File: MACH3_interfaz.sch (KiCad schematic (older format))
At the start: 66 parts, among them J1 USB_B_Micro, J11 Screw_Terminal_01x06, J2 DB25_Male_MountingHoles, J3 Screw_Terminal_01x06, J4 Screw_Terminal_01x13, J5 B4B-XH-A_LF__SN_, J6 B4B-XH-A_LF__SN_, J7 B4B-XH-A_LF__SN_, J8 B4B-XH-A_LF__SN_, J9 B4B-XH-A_LF__SN_, Q1 2N7002, Q2 MMBT2222ALT3G, U1 74HC245, U10 PC817, U2 74HC245, U3 PC817, U4 PC817, U5 PC817, U6 PC817, U7 PC817, U8 LM317MABDTG, U9 LM358

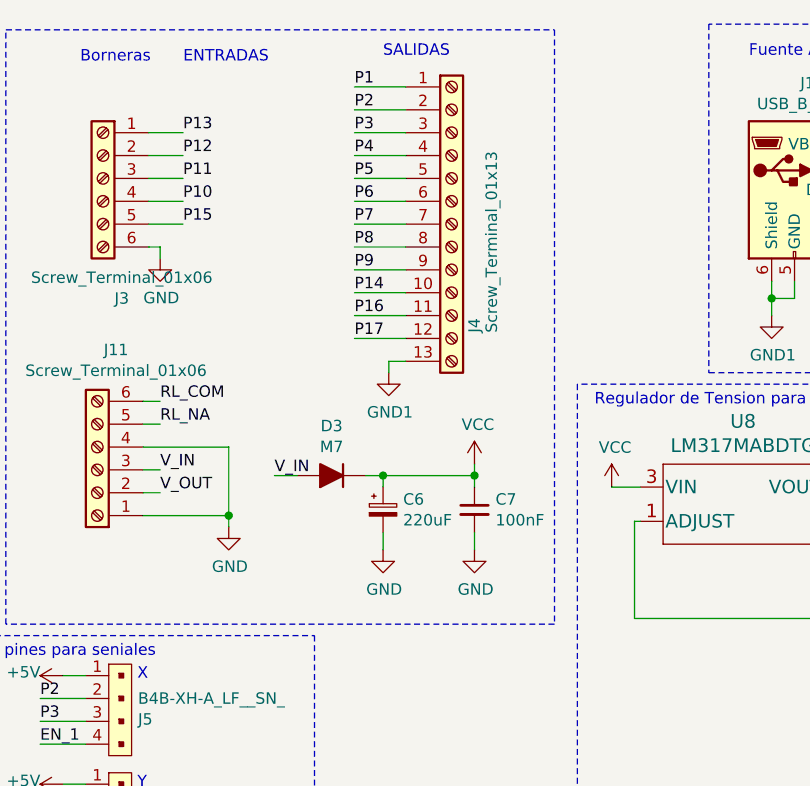
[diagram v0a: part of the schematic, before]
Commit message: Para correccion Docente Eschema, Companiero PCB
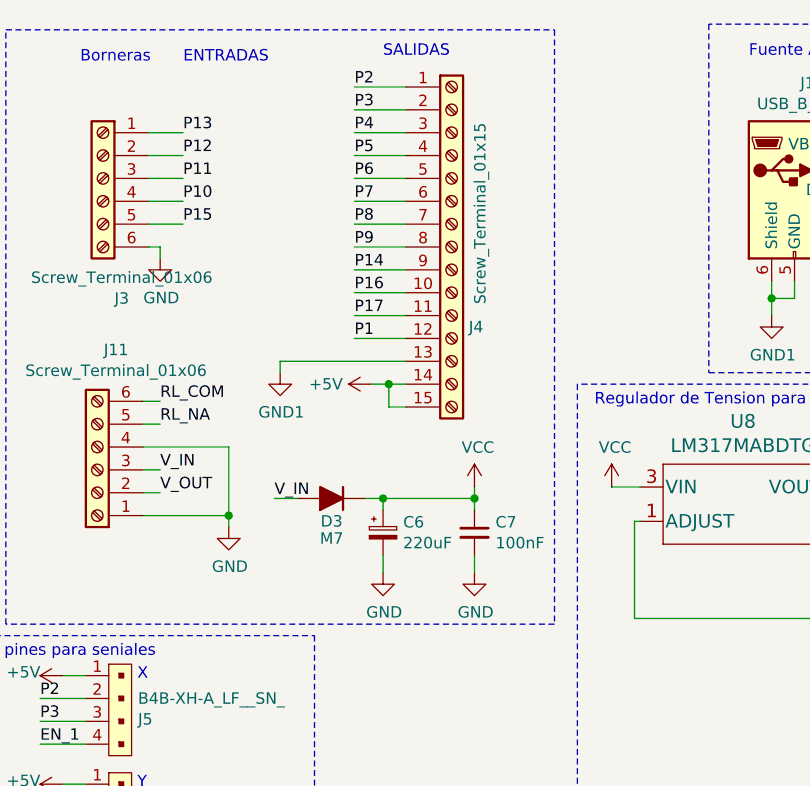
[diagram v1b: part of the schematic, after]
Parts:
- removed J4: Screw_Terminal_01x13, TerminalBlock_Phoenix:TerminalBlock_Phoenix_MKDS-1,5-13_1x13_P5.00mm_Horizontal, symbol Connector:Screw_Terminal_01x13
- added J4: Screw_Terminal_01x15, TerminalBlock_Phoenix:TerminalBlock_Phoenix_MKDS-1,5-15_1x15_P5.00mm_Horizontal, symbol Connector:Screw_Terminal_01x15
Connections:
- net +5V: now also J4.14 (Pin_14), J4.15 (Pin_15)
- net GND1: now also J4.13 (Pin_13)
- net P1: now also J4.12 (Pin_12)
- net P14: now also J4.9 (Pin_9)
- net P16: now also J4.10 (Pin_10)
- net P17: now also J4.11 (Pin_11)
- net P2: now also J4.1 (Pin_1)
- net P3: now also J4.2 (Pin_2)
- net P4: now also J4.3 (Pin_3)
- net P5: now also J4.4 (Pin_4)
- net P6: now also J4.5 (Pin_5)
- net P7: now also J4.6 (Pin_6)
- net P8: now also J4.7 (Pin_7)
- net P9: now also J4.8 (Pin_8)
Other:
- moved on the sheet: C6, C7, D3
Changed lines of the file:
@@
 Text Label 5075 3925 0    50   ~ 0
 P17
-$Comp
-L Connector:Screw_Terminal_01x13 J4
-U 1 1 60736E15
-P 7750 1375
-F 0 "J4" V 7850 900 50  0000 L CNN
-F 1 "Screw_Terminal_01x13" V 7925 900 50  0000 L CNN
-F 2 "TerminalBlock_Phoenix:TerminalBlock_Phoenix_MKDS-1,5-13_1x13_P5.00mm_Horizontal" H 7750 1375 50  0001 C CNN
-F 3 "~" H 7750 1375 50  0001 C CNN
-	1    7750 1375
-	1    0    0    -1
-$EndComp
+Wire Wire Line
+	7550 1875 7325 1875
 Wire Wire Line
 	7550 775  7325 775
@@
 	7550 1775 7325 1775
 Wire Wire Line
-	7550 1875 7325 1875
-Wire Wire Line
-	7550 1975 7475 1975
-Wire Wire Line
-	7475 1975 7475 2025
+	7550 1975 7000 1975
+Wire Wire Line
+	7000 1975 7000 2025
+Text Label 7325 1875 0    50   ~ 0
+P1
 Text Label 7325 775  0    50   ~ 0
-P1
+P2
 Text Label 7325 875  0    50   ~ 0
-P2
+P3
 Text Label 7325 975  0    50   ~ 0
-P3
+P4
 Text Label 7325 1075 0    50   ~ 0
-P4
+P5
 Text Label 7325 1175 0    50   ~ 0
-P5
+P6
 Text Label 7325 1275 0    50   ~ 0
-P6
+P7
 Text Label 7325 1375 0    50   ~ 0
-P7
+P8
 Text Label 7325 1475 0    50   ~ 0
-P8
+P9
 Text Label 7325 1575 0    50   ~ 0
-P9
+P14
 Text Label 7325 1675 0    50   ~ 0
-P14
+P16
 Text Label 7325 1775 0    50   ~ 0
-P16
-Text Label 7325 1875 0    50   ~ 0
 P17
 Text Notes 7450 650  0    50   ~ 0
@@
 $EndComp
 Wire Wire Line
-	7850 2800 7850 2725
+	7850 2900 7850 2825
 $Comp
 L power:GND #PWR0122
 U 1 1 6077A5B8
-P 7850 2800
-F 0 "#PWR0122" H 7850 2550 50  0001 C CNN
-F 1 "GND" H 7855 2627 50  0000 C CNN
-F 2 "" H 7850 2800 50  0001 C CNN
-F 3 "" H 7850 2800 50  0001 C CNN
-	1    7850 2800
-	1    0    0    -1
-$EndComp
-Connection ~ 7450 2475
-Wire Wire Line
-	7850 2475 7450 2475
-Wire Wire Line
-	7850 2525 7850 2475
-Wire Wire Line
-	7450 2475 7450 2525
+P 7850 2900
+F 0 "#PWR0122" H 7850 2650 50  0001 C CNN
+F 1 "GND" H 7855 2727 50  0000 C CNN
+F 2 "" H 7850 2900 50  0001 C CNN
+F 3 "" H 7850 2900 50  0001 C CNN
+	1    7850 2900
+	1    0    0    -1
+$EndComp
+Connection ~ 7450 2575
+Wire Wire Line
+	7850 2575 7450 2575
+Wire Wire Line
+	7850 2625 7850 2575
+Wire Wire Line
+	7450 2575 7450 2625
 $Comp
 L Device:CP_Small C6
 U 1 1 606FAE5F
-P 7450 2625
-F 0 "C6" H 7538 2671 50  0000 L CNN
-F 1 "220uF" H 7538 2580 50  0000 L CNN
-F 2 "Capacitor_THT:CP_Radial_D8.0mm_P3.80mm" H 7450 2625 50  0001 C CNN
-F 3 "~" H 7450 2625 50  0001 C CNN
-	1    7450 2625
+P 7450 2725
+F 0 "C6" H 7538 2771 50  0000 L CNN
+F 1 "220uF" H 7538 2680 50  0000 L CNN
+F 2 "Capacitor_THT:CP_Radial_D8.0mm_P3.80mm" H 7450 2725 50  0001 C CNN
+F 3 "~" H 7450 2725 50  0001 C CNN
+	1    7450 2725
 	1    0    0    -1
 $EndComp
@@
 L power:GND #PWR0123
 U 1 1 6074053C
-P 7450 2800
-F 0 "#PWR0123" H 7450 2550 50  0001 C CNN
-F 1 "GND" H 7455 2627 50  0000 C CNN
-F 2 "" H 7450 2800 50  0001 C CNN
-F 3 "" H 7450 2800 50  0001 C CNN
-	1    7450 2800
-	1    0    0    -1
-$EndComp
-Wire Wire Line
-	7375 2475 7450 2475
+P 7450 2900
+F 0 "#PWR0123" H 7450 2650 50  0001 C CNN
+F 1 "GND" H 7455 2727 50  0000 C CNN
+F 2 "" H 7450 2900 50  0001 C CNN
+F 3 "" H 7450 2900 50  0001 C CNN
+	1    7450 2900
+	1    0    0    -1
+$EndComp
+Wire Wire Line
+	7375 2575 7450 2575
 $Comp
 L Device:D_ALT D3
 U 1 1 606DE50A
-P 7225 2475
-F 0 "D3" H 7225 2258 50  0000 C CNN
-F 1 "M7" H 7225 2349 50  0000 C CNN
-F 2 "Diode_SMD:D_SMA_Handsoldering" H 7225 2475 50  0001 C CNN
-F 3 "~" H 7225 2475 50  0001 C CNN
-	1    7225 2475
+P 7225 2575
+F 0 "D3" H 7225 2675 50  0000 C CNN
+F 1 "M7" H 7225 2750 50  0000 C CNN
+F 2 "Diode_SMD:D_SMA_Handsoldering" H 7225 2575 50  0001 C CNN
+F 3 "~" H 7225 2575 50  0001 C CNN
+	1    7225 2575
 	-1   0    0    1
 $EndComp
@@
 L Device:C_Small C7
 U 1 1 6129BC97
-P 7850 2625
-F 0 "C7" H 7942 2671 50  0000 L CNN
-F 1 "100nF" H 7942 2580 50  0000 L CNN
-F 2 "Capacitor_SMD:C_0805_2012Metric_Pad1.18x1.45mm_HandSolder" H 7850 2625 50  0001 C CNN
-F 3 "~" H 7850 2625 50  0001 C CNN
-	1    7850 2625
+P 7850 2725
+F 0 "C7" H 7942 2771 50  0000 L CNN
+F 1 "100nF" H 7942 2680 50  0000 L CNN
+F 2 "Capacitor_SMD:C_0805_2012Metric_Pad1.18x1.45mm_HandSolder" H 7850 2725 50  0001 C CNN
+F 3 "~" H 7850 2725 50  0001 C CNN
+	1    7850 2725
 	1    0    0    -1
 $EndComp
@@
 L power:GND1 #PWR0105
 U 1 1 626D01A2
-P 7475 2025
-F 0 "#PWR0105" H 7475 1775 50  0001 C CNN
-F 1 "GND1" H 7480 1852 50  0000 C CNN
-F 2 "" H 7475 2025 50  0001 C CNN
-F 3 "" H 7475 2025 50  0001 C CNN
-	1    7475 2025
+P 7000 2025
+F 0 "#PWR0105" H 7000 1775 50  0001 C CNN
+F 1 "GND1" H 7005 1852 50  0000 C CNN
+F 2 "" H 7000 2025 50  0001 C CNN
+F 3 "" H 7000 2025 50  0001 C CNN
+	1    7000 2025
 	1    0    0    -1
 $EndComp
@@
 	9950 3025 9950 2925
 Wire Wire Line
-	7450 2800 7450 2725
+	7450 2900 7450 2825
 Wire Wire Line
 	6475 1475 6475 1525
@@
 L power:VCC #PWR0144
 U 1 1 629C176A
-P 7850 2425
-F 0 "#PWR0144" H 7850 2275 50  0001 C CNN
-F 1 "VCC" H 7865 2598 50  0000 C CNN
-F 2 "" H 7850 2425 50  0001 C CNN
-F 3 "" H 7850 2425 50  0001 C CNN
-	1    7850 2425
+P 7850 2525
+F 0 "#PWR0144" H 7850 2375 50  0001 C CNN
+F 1 "VCC" H 7865 2698 50  0000 C CNN
+F 2 "" H 7850 2525 50  0001 C CNN
+F 3 "" H 7850 2525 50  0001 C CNN
+	1    7850 2525
 	1    0    0    -1
 $EndComp
@@
 $EndComp
 Wire Wire Line
-	7850 2425 7850 2475
-Connection ~ 7850 2475
+	7850 2525 7850 2575
+Connection ~ 7850 2575
 $Comp
 L power:VCC #PWR0146
@@
 	6400 2450 6475 2450
 Wire Wire Line
-	7075 2475 6975 2475
+	7075 2575 6975 2575
 Text Label 6475 2450 0    50   ~ 0
 V_IN
-Text Label 6975 2475 0    50   ~ 0
+Text Label 6975 2575 0    50   ~ 0
 V_IN
 Wire Notes Line
@@
 	1    0    0    -1
 $EndComp
+$Comp
+L Connector:Screw_Terminal_01x15 J4
+U 1 1 60952780
+P 7750 1475
+F 0 "J4" H 7825 1125 50  0000 L CNN
+F 1 "Screw_Terminal_01x15" V 7875 1225 50  0000 L CNN
+F 2 "TerminalBlock_Phoenix:TerminalBlock_Phoenix_MKDS-1,5-15_1x15_P5.00mm_Horizontal" H 7750 1475 50  0001 C CNN
+F 3 "~" H 7750 1475 50  0001 C CNN
+	1    7750 1475
+	1    0    0    -1
+$EndComp
+$Comp
+L power:+5V #PWR0148
+U 1 1 60997041
+P 7400 2075
+F 0 "#PWR0148" H 7400 1925 50  0001 C CNN
+F 1 "+5V" V 7400 2275 50  0000 C CNN
+F 2 "" H 7400 2075 50  0001 C CNN
+F 3 "" H 7400 2075 50  0001 C CNN
+	1    7400 2075
+	0    -1   -1   0
+$EndComp
+Wire Wire Line
+	7400 2075 7475 2075
+Wire Wire Line
+	7550 2175 7475 2175
+Wire Wire Line
+	7475 2175 7475 2075
+Connection ~ 7475 2075
+Wire Wire Line
+	7475 2075 7550 2075
 $EndSCHEMATC

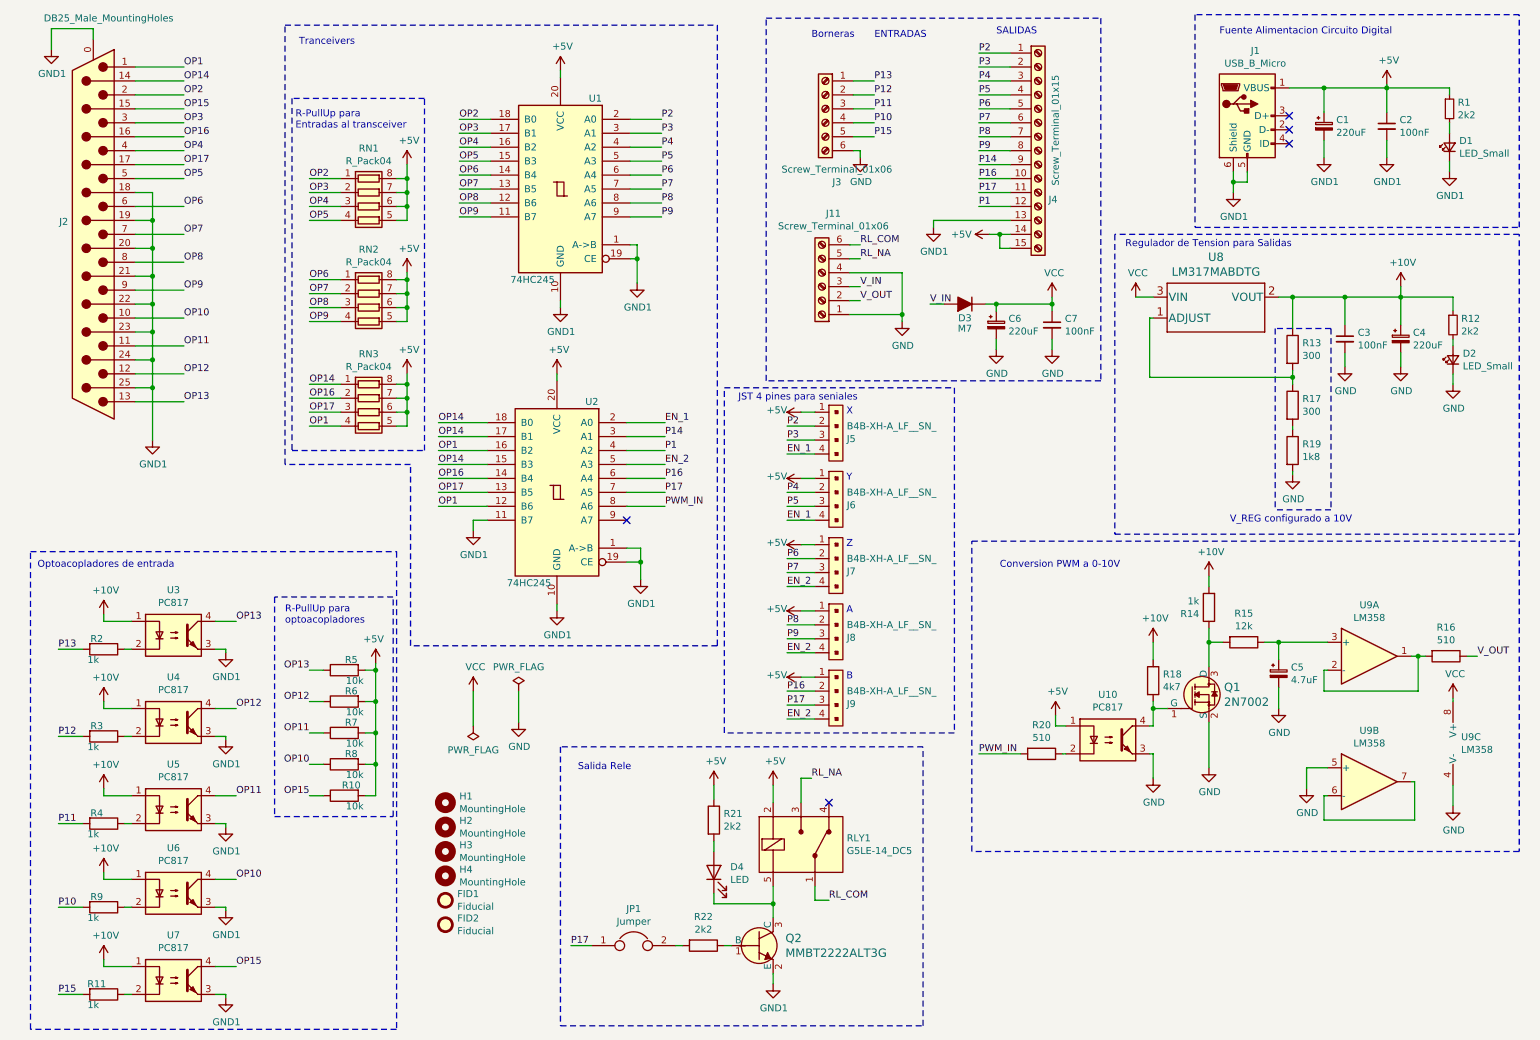
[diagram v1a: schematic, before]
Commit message: Listo para revision final
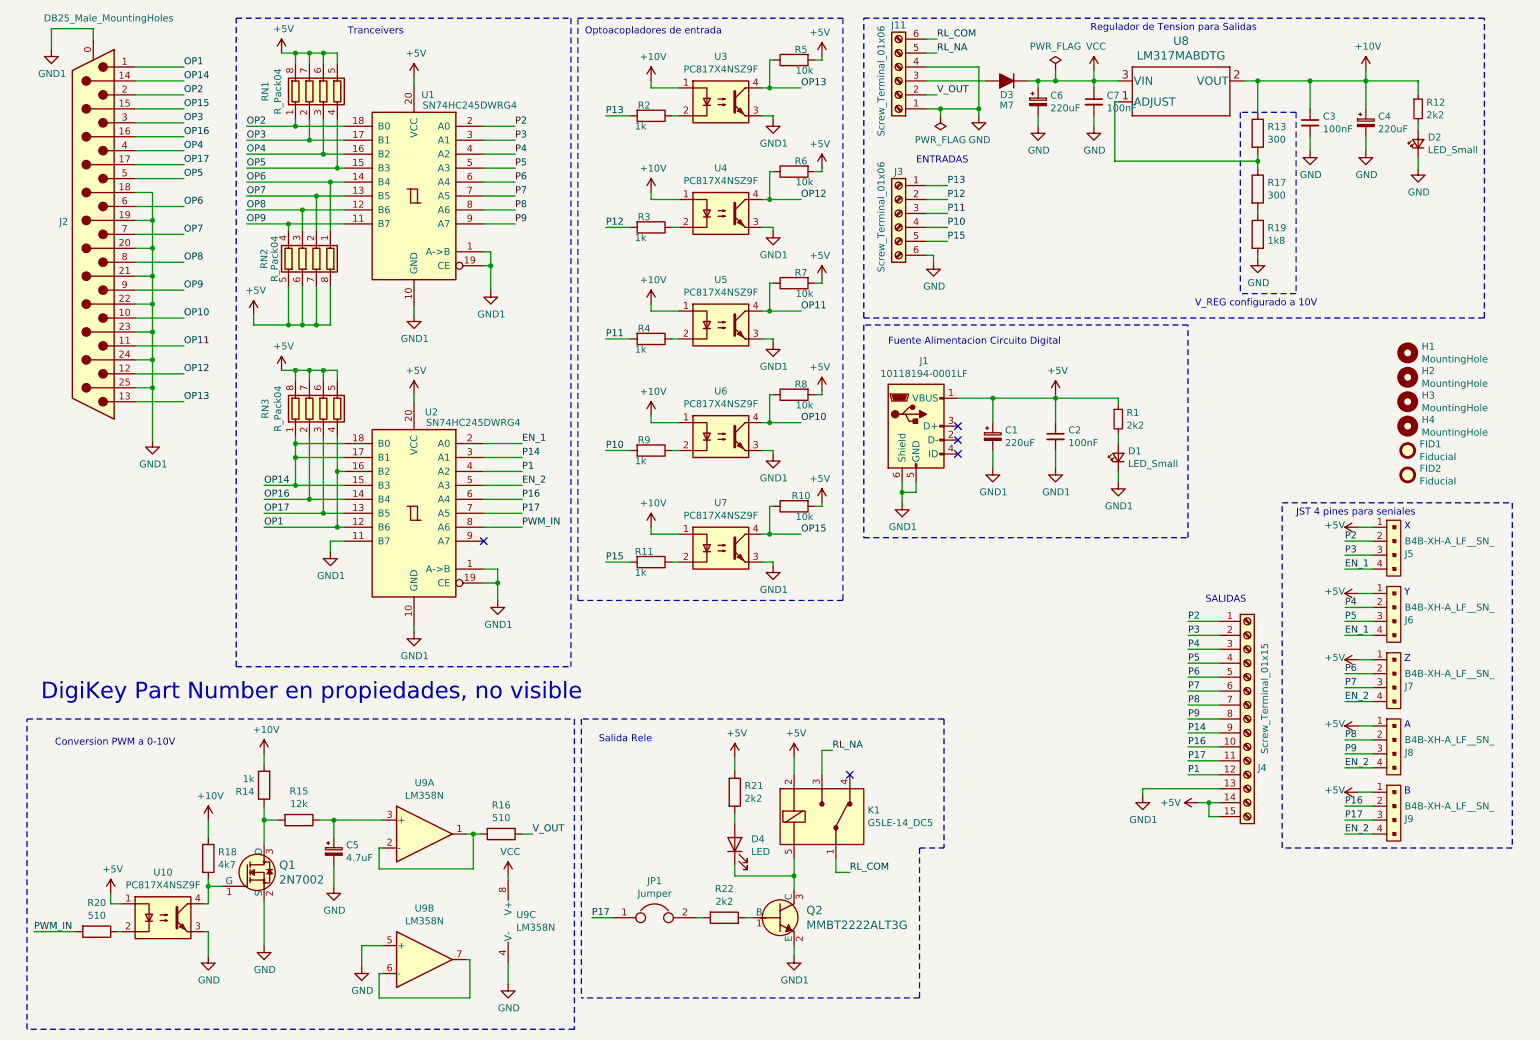
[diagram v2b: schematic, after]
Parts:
- J1: value USB_B_Micro -> 10118194-0001LF; DigiKey (none) -> 609-4618-2-ND - Tape & Reel (TR)
- K1: renamed from RLY1; DigiKey (none) -> Z1011-ND
- U1, U2: value 74HC245 -> SN74HC245DWRG4; DigiKey (none) -> 296-52721-2-ND - Tape & Reel (TR)
- U10, U3, U4, U5, U6, U7: value PC817 -> PC817X4NSZ9F; DigiKey (none) -> PC817X4NSZ9F-ND
- U8: DigiKey (none) -> LM317MABDTG-ND
- U9: value LM358 -> LM358N; DigiKey (none) -> 2156-LM358N-ND
- U9: value LM358 -> LM358N
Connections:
- net V_IN: no longer names the net of D3.2 (A), J11.3 (Pin_3)
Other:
- note added: "DigiKey Part Number en propiedades, no visible"
- note removed: "Borneras"
- note removed: "R-PullUp para \noptoacopladores"
- note removed: "R-PullUp para\nEntradas al transceiver"
- moved on the sheet: C1, C2, C3, C4, C5, C6, C7, D1, D2, D3, D4, FID1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
